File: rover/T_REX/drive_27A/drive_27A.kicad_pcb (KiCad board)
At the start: 4 copper layers, 30 x 58.2 mm, 54 parts, among them J1 USB_B_Micro, J2 RJ45, J6 XT30PW-M, J7 XT30PW-F, J9 B4B-XH-A_LF__SN_, SW1 TS09-63-25-WT-160-SMT-TR, SW2 TS09-63-25-WT-160-SMT-TR, U2 TJA1050T_CM_118, U3 AZ1117ID-3.3TRG1, U4 BTN8962TA, U5 BTN8962TA, U6 ESP32-S3-WROOM-1

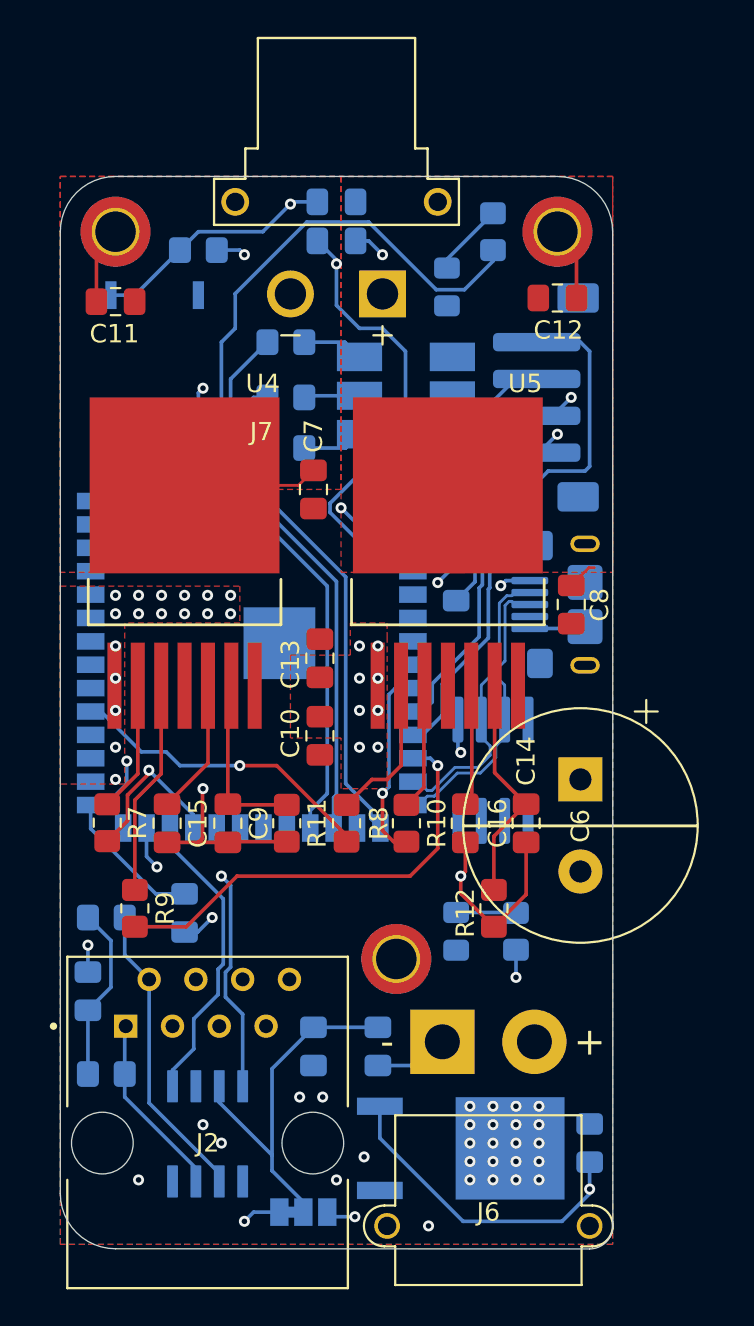
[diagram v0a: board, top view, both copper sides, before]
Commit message: .
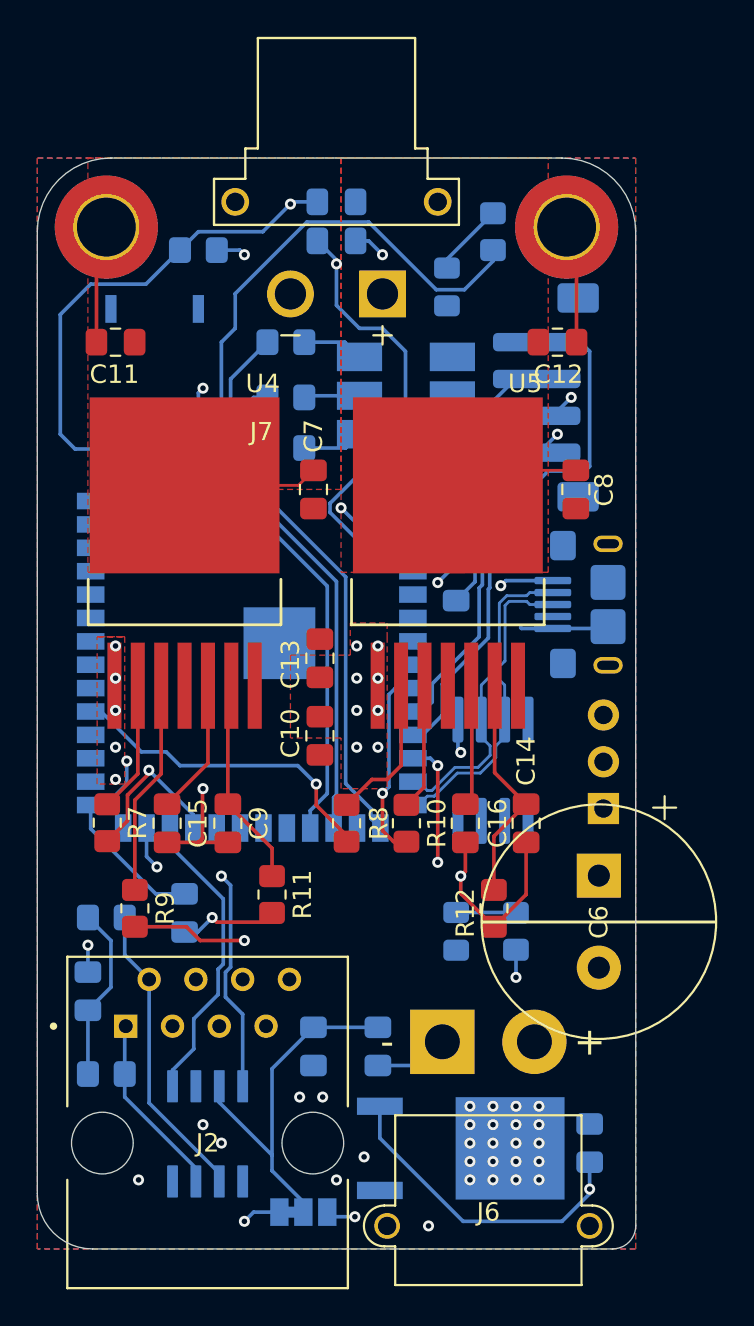
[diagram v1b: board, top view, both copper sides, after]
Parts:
- removed H3: MountingHole_Pad, MountingHole:MountingHole_2.2mm_M2_DIN965_Pad_TopBottom
- added JP1: Jumper_3_Open, Connector_PinHeader_2.54mm:PinHeader_1x03_P2.54mm_Vertical, B.Cu at (45.0, 49.8)
- H1, H2: footprint MountingHole:MountingHole_2.2mm_M2_DIN965_Pad_TopBottom -> MountingHole:MountingHole_3.2mm_M3_DIN965_Pad_TopBottom
- U2: value TJA1050T_CM_118 -> SN65HVD232Q
- moved C8 6.25 mm to (43.5, 32.5)
- moved C6 5.32 mm to (44.8, 53.5)
- moved R11 3.95 mm to (27.0, 54.5)
- moved C12 2.40 mm to (42.5, 24.5)
- moved C11 2.20 mm to (18.5, 24.5)
- moved J1 1.25 mm to (45.2, 38.8)
- moved SW1 0.75 mm to (18.2, 26.5), turned to -90 degrees
- moved SW2 0.75 mm to (23.0, 26.5)
- moved H1 0.56 mm to (18.0, 18.2)
- moved H2 0.56 mm to (43.0, 18.2)
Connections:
- C3 pad 1: Net-(JP1-C) -> +3.3V
- C4 pad 1: Net-(JP1-C) -> +3.3V
- C5 pad 1: +5V -> Net-(JP1-C)
- J9 pad : GND -> (no net)
- U2 pad 3: Net-(JP1-C) -> +3.3V
- U3 pad 1: GND -> unconnected-(U3-GND-Pad1)
- U3 pad 2: +3.3V -> unconnected-(U3-OUTPUT-Pad2)
- U3 pad 3: +5V -> unconnected-(U3-INPUT-Pad3)
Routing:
- net EN_PB: track 42.3 -> 55.1 mm
- net J2-: track 1.65 -> 7.04 mm
- net GND: track 45.1 -> 49.4 mm, vias 40 -> 28
- net J2_EN_1: track 24.2 -> 26.0 mm, vias 1 -> 3
- net Net-(U4-IS): track 9.73 -> 11.4 mm
- net USB_N: track 15.9 -> 17.2 mm
- net USB_P: track 15.9 -> 17.2 mm
- net +5V: track 85.9 -> 87.2 mm
- net +24V: track 0.71 -> 0.00 mm
- net J2_IN_2: track 17.0 -> 17.7 mm
- net LED_BUILDIN: track 36.4 -> 37.0 mm
- net unconnected-(U3-OUTPUT-Pad2): vias 0 -> 20
- net +3.3V: vias 25 -> 5
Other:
- board size 30 x 58.2 mm -> 32.5 x 59.3 mm

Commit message: rev3 drive27A
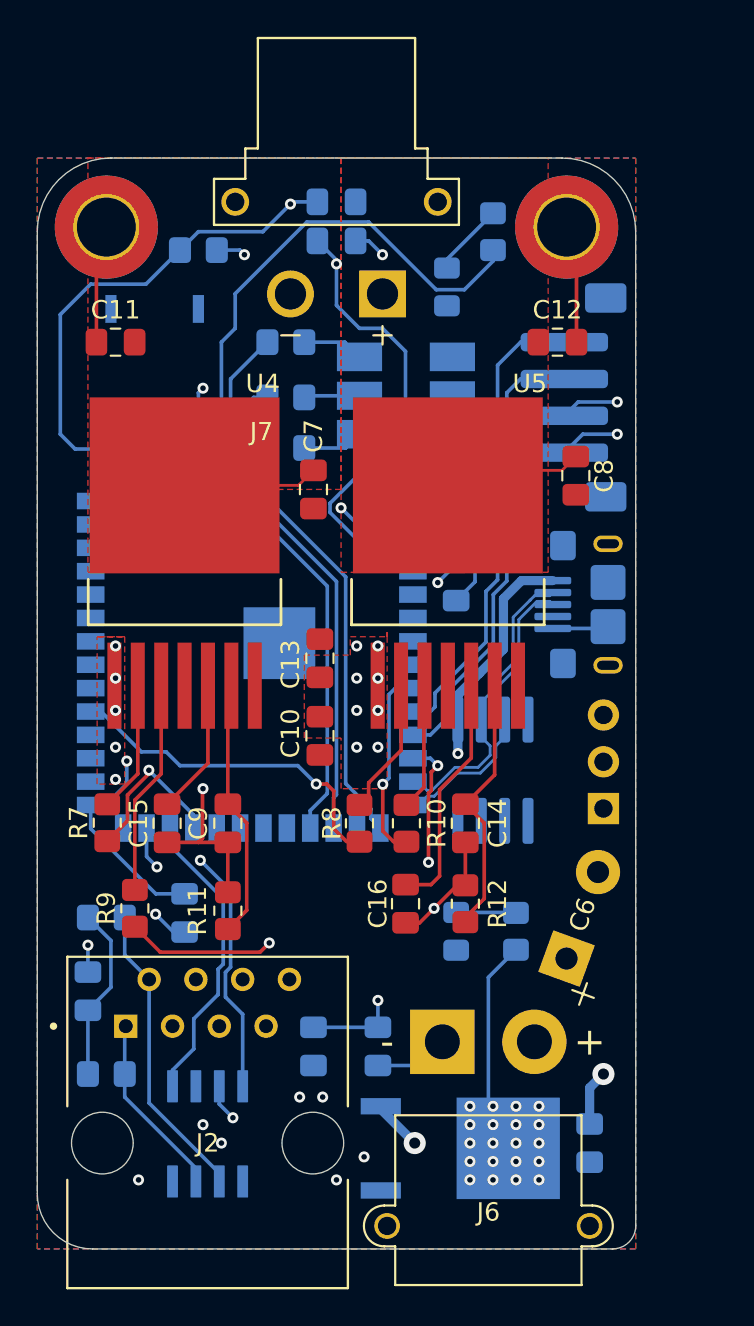
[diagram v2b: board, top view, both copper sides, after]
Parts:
- removed the JP1 at (28.7, 71.8)
- U3: value AZ1117ID-3.3TRG1 -> LD1086DT33TR; footprint LDO_AZ1117ID-3.3TRG1:TO252-2_AZ1117ID-3.3TRG1_DIO -> LDO_AZ1117ID-3.3TRG1:TO252-2_AZ1117ID-3.3TRG1_DIO-L
- moved C16 5.45 mm to (34.2, 55.0)
- moved C6 4.84 mm to (43.0, 58.0), turned to 70 degrees
- moved C14 3.30 mm to (37.5, 50.6)
- moved R11 2.56 mm to (24.6, 55.4), turned to 90 degrees
- moved R12 1.57 mm to (37.5, 55.0), turned to 90 degrees
- moved J9 1.50 mm to (43.8, 27.5)
- moved C8 0.75 mm to (43.5, 31.8)
- moved R8 0.70 mm to (31.8, 50.6)
- turned C5 to -90 degrees
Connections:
- U3 pad 1: unconnected-(U3-GND-Pad1) -> GND
- U3 pad 2: unconnected-(U3-OUTPUT-Pad2) -> +3.3V
- U3 pad 3: unconnected-(U3-INPUT-Pad3) -> Net-(JP1-C)
- U6 pad 10: ENC_QUAD_A -> ENC_QUAD_B
- U6 pad 11: ENC_QUAD_B -> ENC_QUAD_A
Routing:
- net Net-(JP1-C): track 20.1 -> 46.5 mm, vias 0 -> 2
- net +3.3V: track 18.3 -> 35.5 mm, vias 5 -> 25
- net +5V: track 87.2 -> 79.9 mm, vias 4 -> 1
- net Net-(U5-SR): track 6.59 -> 13.1 mm
- net GND: track 49.4 -> 44.6 mm, vias 28 -> 27
- net ENC_QUAD_B: track 29.4 -> 25.4 mm
- net Net-(U4-IS): track 11.4 -> 14.1 mm
- net ENC_QUAD_A: track 22.2 -> 24.7 mm
- net Net-(U5-IS): track 12.5 -> 14.3 mm
- net USB_P: track 17.2 -> 16.3 mm
- net USB_N: track 17.2 -> 16.3 mm
- net Net-(U5-IN): track 8.18 -> 7.41 mm
- net J2-: track 7.04 -> 7.60 mm
- net J2_EN_1: track 26.0 -> 26.5 mm
- net unconnected-(U3-OUTPUT-Pad2): vias 20 -> 0
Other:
- board text added: "*"
- board text added: "Prog"
- board text removed: "3.3V"
- board text removed: "5V"
